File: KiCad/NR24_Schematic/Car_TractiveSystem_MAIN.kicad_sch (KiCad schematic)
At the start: 19 parts, among them J1 M_con, J2 F_con, K2 Key Switch Relay, M1 Zero_7R_Motor, SW1 12V E-stop, SW3 GLVMS, SW4 Break Over Travel, SW7 TSMS, SW8 12V E-stop, U1 Sevcon_Gen4_Size6, U2 Throttle, U4 Vehicle Dynamic Module, U6 AEMnet_Logger, U7 Brake Pressure Sensor (Aim)

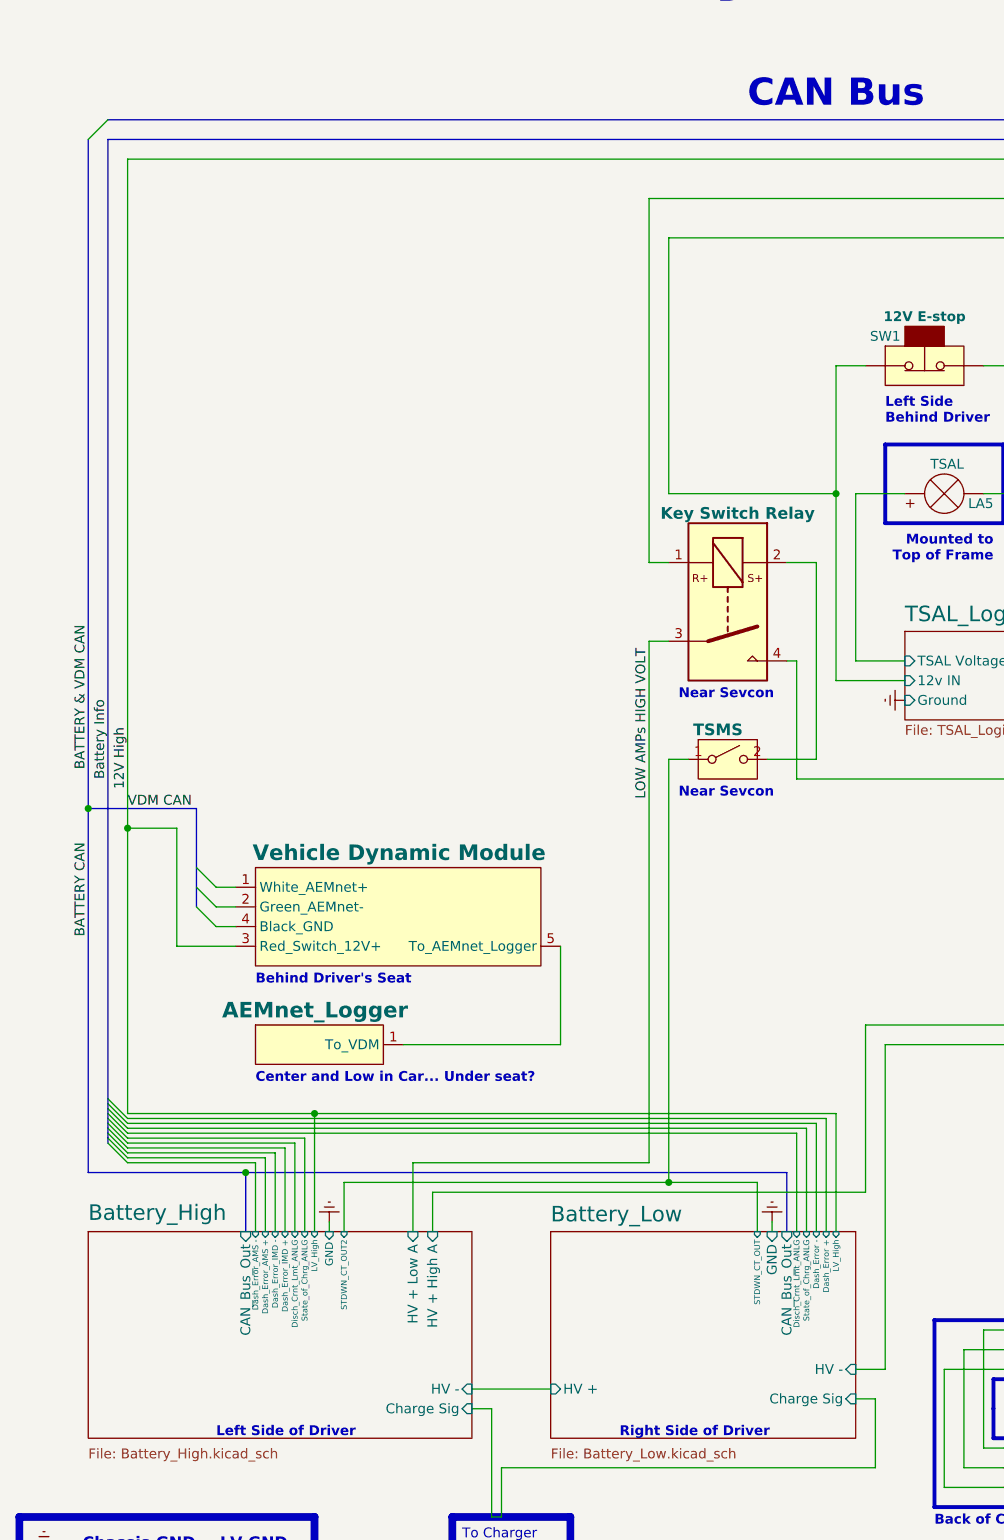
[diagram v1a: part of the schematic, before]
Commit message: first iteration
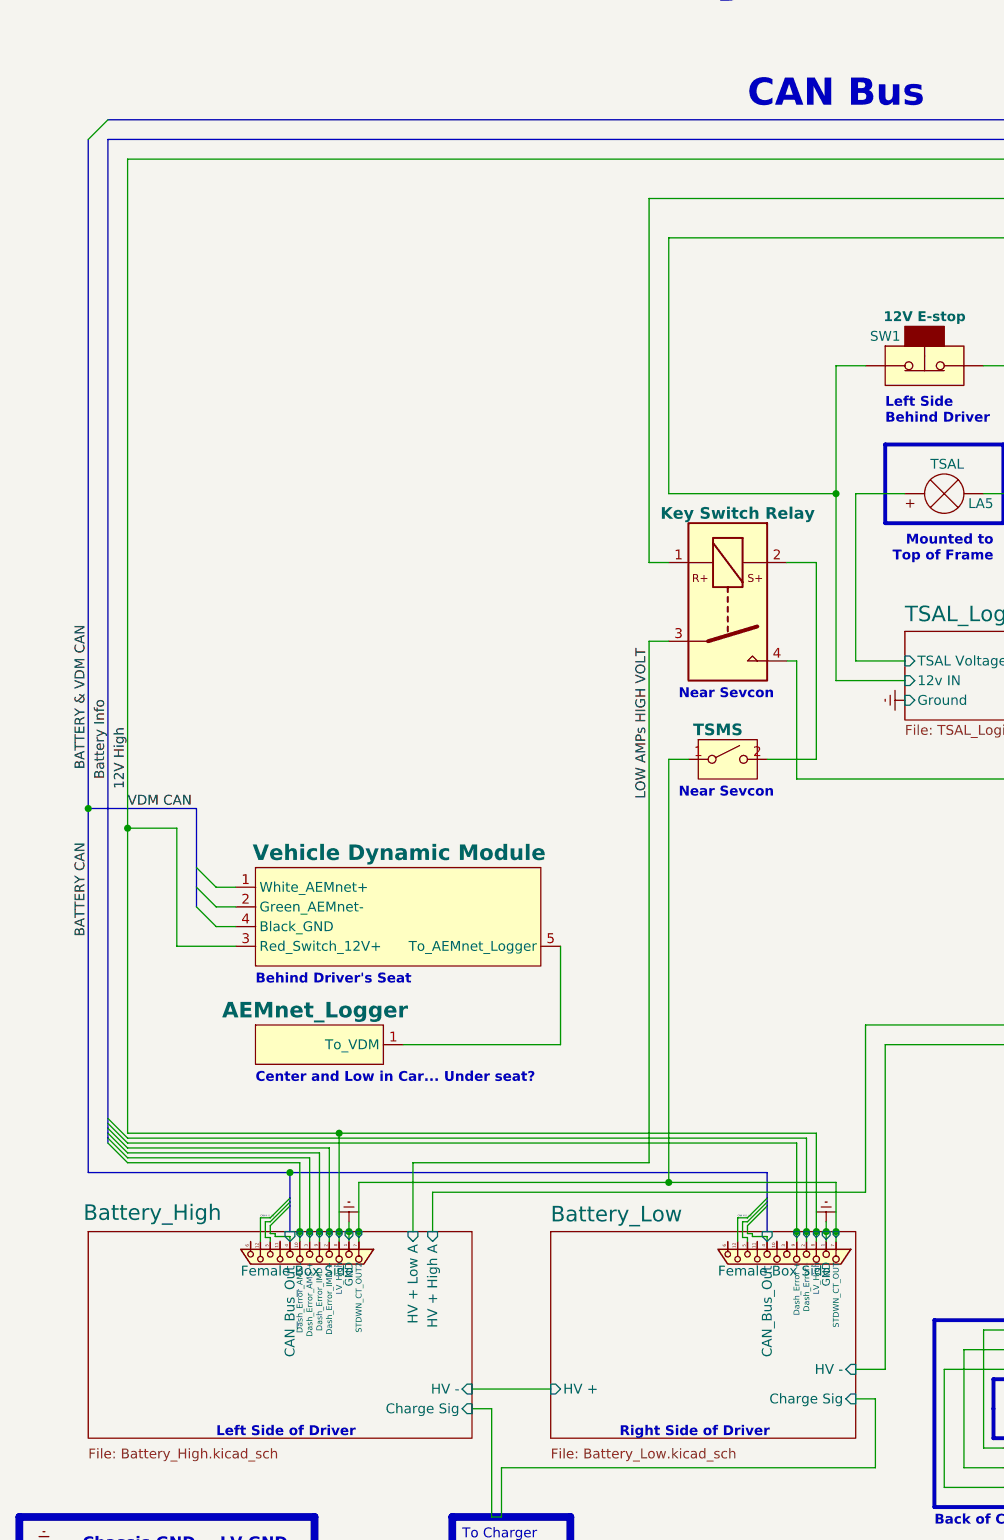
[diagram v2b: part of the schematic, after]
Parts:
- added J3, J4: Female Box Side, symbol Connector:DA15_Receptacle
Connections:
- net  VDM CAN: now also J3.8, J4.8
- net Earth: now also J3.1, J4.1
- net Battery_High/STDWN_CT_OUT2 renamed Battery_High/STDWN_CT_OUT2         
- net Battery_High/STDWN_CT_OUT2         : now also J3.7, J4.7
- new net Battery_High/Dash_Error_AMS +         : J3.3
- new net Battery_High/Dash_Error_AMS -         : J3.10 (P10)
- new net Battery_High/Dash_Error_IMD +         : J3.2
- new net Battery_High/Dash_Error_IMD -         : J3.9 (P9)
- new net Battery_Low/Dash_Error +         : J4.9 (P9)
- new net Battery_Low/Dash_Error -         : J4.2
- new net CAN H / L / G: J3.12 (P12), J4.12 (P12)
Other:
- sheet Battery_High ports: added CAN_Bus_Out     , Dash_Error_AMS +         , Dash_Error_AMS -         , Dash_Error_IMD +         , Dash_Error_IMD -         , GND      , LV_High         , STDWN_CT_OUT2         ; removed CAN_Bus_Out, Dash_Error_AMS +, Dash_Error_AMS -, Dash_Error_IMD +, Dash_Error_IMD -, Disch_Crnt_Lmt_ANLG, GND, LV_High, STDWN_CT_OUT2, State_of_Chrg_ANLG
- sheet Battery_Low ports: added CAN_Bus_Out     , Dash_Error +         , Dash_Error -         , GND      , LV_High         , STDWN_CT_OUT         ; removed CAN_Bus_Out, Dash_Error +, Dash_Error -, Disch_Crnt_Lmt_ANLG, GND, LV_High, STDWN_CT_OUT, State_of_Chrg_ANLG
